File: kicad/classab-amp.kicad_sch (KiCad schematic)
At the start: 68 parts, among them J1 SPEAKER, J3 INPUT, Q1 BC547, Q10 MJL3281C, Q11 BD140, Q12 MJL1302C, Q13 BC547, Q14 BC557, Q2 BC547, Q3 BC557, Q4 BC557, Q5 BC547, Q6 BD140, Q7 BD139, Q8 BD139, Q9 BD139

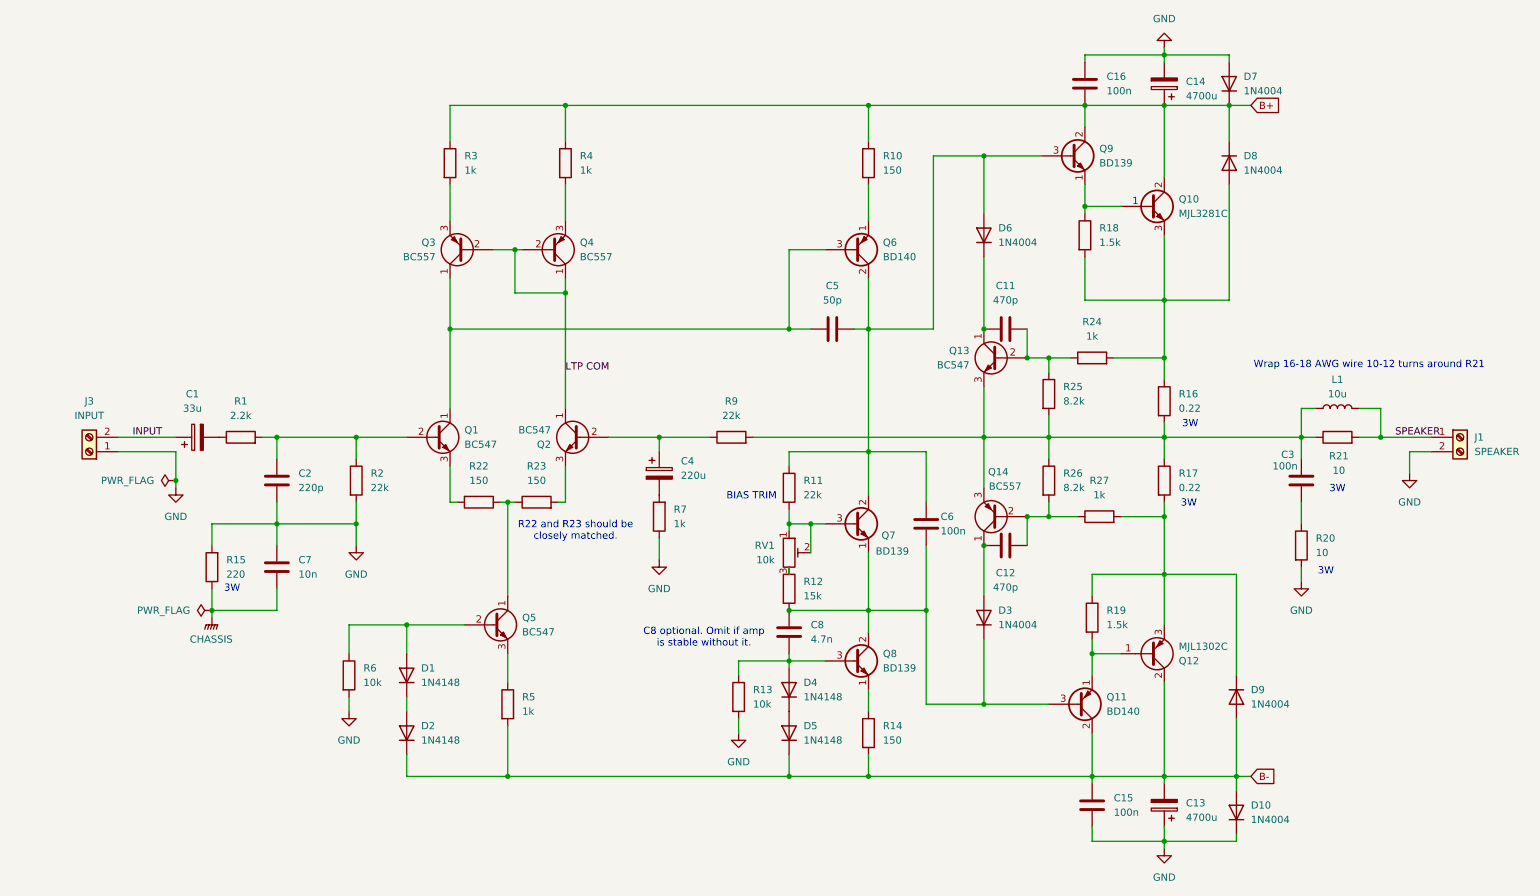
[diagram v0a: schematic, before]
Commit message: Production candidate
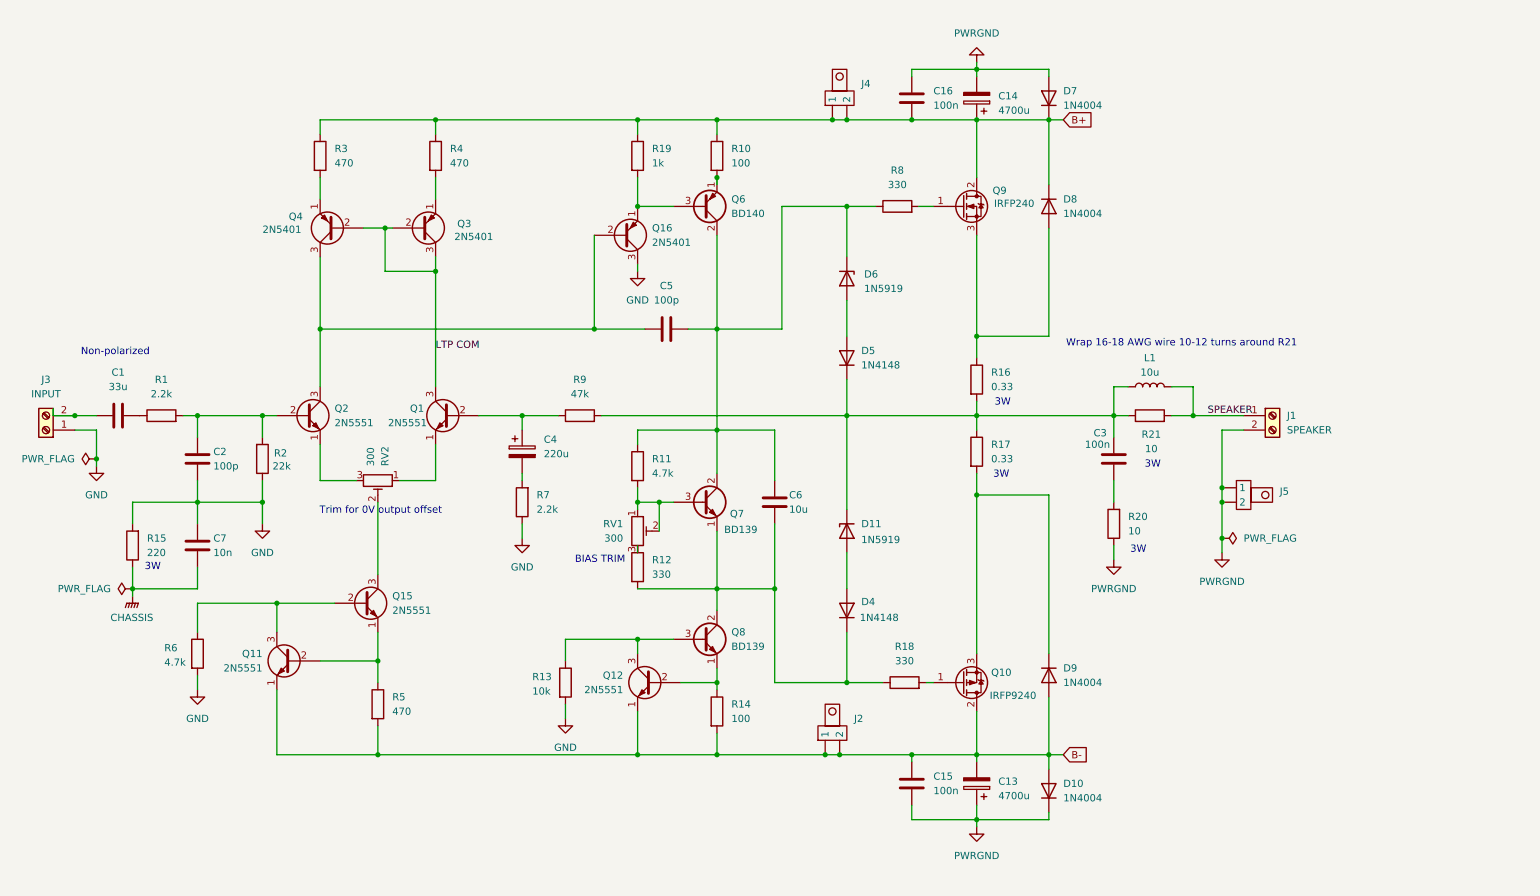
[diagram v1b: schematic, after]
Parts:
- removed C1: 33u, Capacitor_THT:CP_Radial_D4.0mm_P1.50mm, symbol Device:C_Polarized
- removed C11, C12: 470p, Capacitor_THT:C_Rect_L7.2mm_W3.0mm_P5.00mm_FKS2_FKP2_MKS2_MKP2, symbol Device:C
- removed C8: 4.7n, Capacitor_THT:C_Rect_L7.2mm_W3.0mm_P5.00mm_FKS2_FKP2_MKS2_MKP2, symbol Device:C
- removed D1, D2: 1N4148, Diode_THT:D_DO-35_SOD27_P7.62mm_Horizontal, symbol Diode:1N4148
- removed D3, D6: 1N4004, Diode_THT:D_DO-41_SOD81_P10.16mm_Horizontal, symbol Diode:1N4004
- removed Q1, Q13, Q2, Q5: BC547, Package_TO_SOT_THT:TO-92_Inline, symbol Transistor_BJT:BC547
- removed Q10: MJL3281C, Package_TO_SOT_THT:TO-264-3_Vertical, symbol Custom:MJL3218C
- removed Q11: BD140, Package_TO_SOT_THT:TO-126-3_Vertical, symbol Transistor_BJT:BD140
- removed Q12: MJL1302C, Package_TO_SOT_THT:TO-264-3_Vertical, symbol Custom:MJL1302C
- removed Q14, Q3, Q4: BC557, Package_TO_SOT_THT:TO-92_Inline, symbol Transistor_BJT:BC557
- removed Q9: BD139, Package_TO_SOT_THT:TO-126-3_Vertical, symbol Transistor_BJT:BD139
- removed R22, R23: 150, Resistor_THT:R_Axial_DIN0204_L3.6mm_D1.6mm_P7.62mm_Horizontal, symbol Device:R
- removed R24, R27: 1k, Resistor_THT:R_Axial_DIN0204_L3.6mm_D1.6mm_P7.62mm_Horizontal, symbol Device:R
- removed R25, R26: 8.2k, Resistor_THT:R_Axial_DIN0204_L3.6mm_D1.6mm_P7.62mm_Horizontal, symbol Device:R
- added C1: 33u, Capacitor_THT:CP_Radial_D4.0mm_P2.00mm, symbol Device:C
- added D11, D6: 1N5919, Diode_THT:D_DO-41_SOD81_P10.16mm_Horizontal, symbol Device:D_Zener
- added J2, J4, J5: ~, footprints:Spade Connector, symbol Custom:Spade_Connector
- added Q1, Q11, Q12, Q15, Q2: 2N5551, Package_TO_SOT_THT:TO-92_Wide, symbol Custom:2N5551
- added Q10: IRFP9240, Package_TO_SOT_THT:TO-247-3_Vertical, symbol Custom:IRFP9240
- added Q16, Q3, Q4: 2N5401, Package_TO_SOT_THT:TO-92_Wide, symbol Custom:2N5401
- added Q9: IRFP240, Package_TO_SOT_THT:TO-247-3_Vertical, symbol Custom:IRFP240
- added R8: 330, Resistor_THT:R_Axial_DIN0204_L3.6mm_D1.6mm_P7.62mm_Horizontal, symbol Device:R
- added RV2: 300, footprints:TRIM_T93YA103KT20, symbol Device:R_Potentiometer_Trim
- C2: value 220p -> 100p
- C5: value 50p -> 100p
- C6: value 100n -> 10u; footprint Capacitor_THT:C_Rect_L7.2mm_W3.0mm_P5.00mm_FKS2_FKP2_MKS2_MKP2 -> Capacitor_THT:CP_Radial_D4.0mm_P2.00mm
- R1, R2: footprint Resistor_THT:R_Axial_DIN0204_L3.6mm_D1.6mm_P7.62mm_Horizontal -> Resistor_THT:R_Axial_DIN0207_L6.3mm_D2.5mm_P2.54mm_Vertical
- R10, R14: value 150 -> 100
- R11: value 22k -> 4.7k; footprint Resistor_THT:R_Axial_DIN0204_L3.6mm_D1.6mm_P7.62mm_Horizontal -> Resistor_THT:R_Axial_DIN0207_L6.3mm_D2.5mm_P2.54mm_Vertical
- R12: value 15k -> 330; footprint Resistor_THT:R_Axial_DIN0204_L3.6mm_D1.6mm_P7.62mm_Horizontal -> Resistor_THT:R_Axial_DIN0207_L6.3mm_D2.5mm_P2.54mm_Vertical
- R16, R17: value 0.22 -> 0.33
- R18: value 1.5k -> 330
- R19: value 1.5k -> 1k
- R20: footprint Resistor_THT:R_Axial_DIN0414_L11.9mm_D4.5mm_P15.24mm_Horizontal -> Resistor_THT:R_Axial_DIN0516_L15.5mm_D5.0mm_P5.08mm_Vertical
- R3, R4, R5: value 1k -> 470
- R6: value 10k -> 4.7k
- R7: value 1k -> 2.2k
- R9: value 22k -> 47k
- RV1: value 10k -> 300
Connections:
- net B+: now also R19.1, J4.1, J4.2, Q9.2 (D)
- net B-: now also J2.1, J2.2, Q10.2 (D), Q11.1 (E), Q12.1 (E); no longer D5.1 (K)
- net GND: now also R2.1, Q16.3 (C); no longer C13.1, C14.2, C15.2, C16.1, D10.1 (K), D7.2 (A), J1.2 (Pin_2), R2.2, R20.2
- net LTP COM: now also Q1.3 (C), Q3.2 (B), Q3.3 (C), Q4.2 (B)
- net at C6.2, Q7.1 (E), Q8.2 (C)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: now also D4.1 (K), R18.1
- net at D8.2 (A), R16.1: now also Q9.3 (S); no longer R18.2
- net at C3.1, L1.1, R16.2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: now also D5.1 (K), D11.1 (K)
- net at C5.2, C6.1, Q6.2 (C)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: now also D6.1 (K), R8.1
- net at C5.1: now also Q16.2 (B), Q2.3 (C), Q4.3 (C); no longer Q6.3 (B)
- net at D9.1 (K), R17.2: now also Q10.3 (S); no longer R19.1
- net at D5.2 (A): now also D6.2 (A); no longer D4.1 (K)
- net at Q8.3 (B), R13.1: now also Q12.3 (C); no longer D4.2 (A)
- net at R19.2: now also Q6.3 (B), Q16.1 (E)
- net at C2.1, R1.2: now also R2.2, Q2.2 (B); no longer R2.1
- net at R3.2: now also Q4.1 (E)
- net at R6.1: now also Q11.3 (C), Q15.2 (B)
- net at Q8.1 (E), R14.1: now also Q12.2 (B)
- net at C4.1, R9.1: now also Q1.2 (B)
- net at R5.1: now also Q11.2 (B), Q15.1 (E)
- net at R4.2: now also Q3.1 (E)
- net at C3.2: now also R20.2; no longer R20.1
- net at R1.1: now also C1.2
- net INPUT: no longer names the net of J3.2 (Pin_2)
- net INPUT: now also C1.1
- new net: Q1.1 (E), RV2.1
- new net: Q15.3 (C), RV2.2
- new net: Q2.1 (E), RV2.3
- new net: Q9.1 (G), R8.2
- new net: D11.2 (A), D4.2 (A)
- new net: Q10.1 (G), R18.2
- new net PWRGND: C13.1, C14.2, C15.2, C16.1, D10.1 (K), D7.2 (A), J1.2 (Pin_2), J5.1, J5.2, R20.1
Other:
- note added: "Non-polarized"
- note added: "Trim for 0V output offset"
- note removed: "C8 optional. Omit if amp is stable without it."
- note removed: "R22 and R23 should be closely matched."
- moved on the sheet: C13, C14, C15, C16, C2, C3, C4, C5, C6, C7, D10, D7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
